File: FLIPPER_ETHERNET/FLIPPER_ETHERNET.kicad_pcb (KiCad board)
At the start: 2 copper layers, 67 x 25 mm, 38 parts, among them J1 RJ45_Hanrun_HR911105A_Horizon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, J2 Conn_01x08_Socket, J3 Conn_01x10_Socket, SW1 SW_Push, U1 ENC28J60x-ML, Y1 25MHz

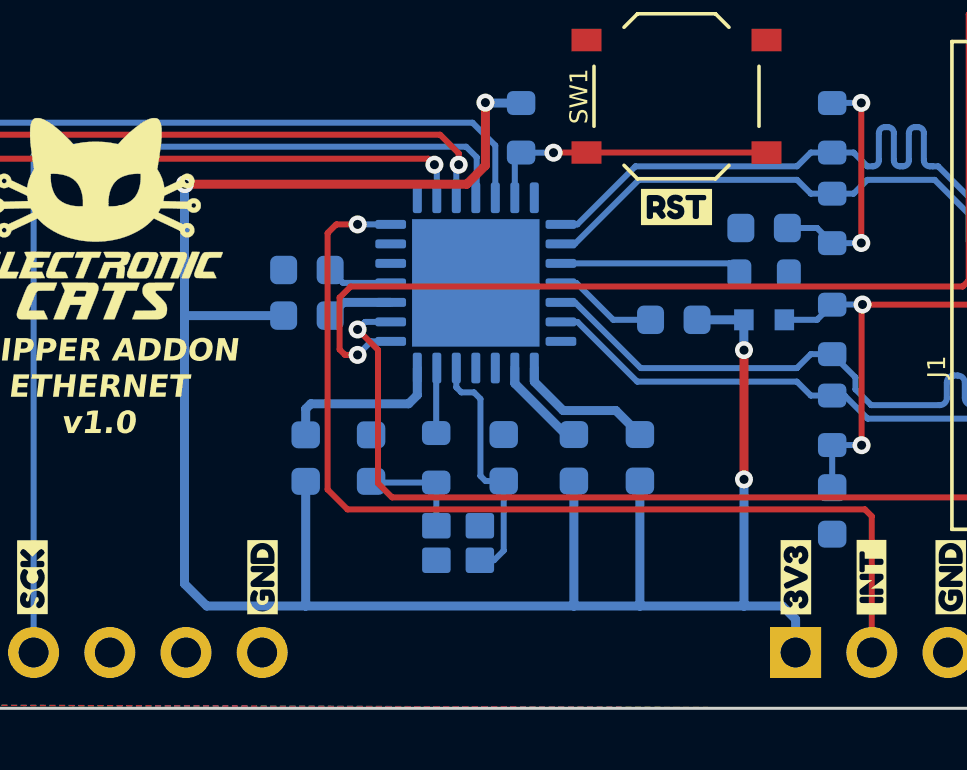
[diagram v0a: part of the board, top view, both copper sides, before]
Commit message: feat: some pcb routes corrected
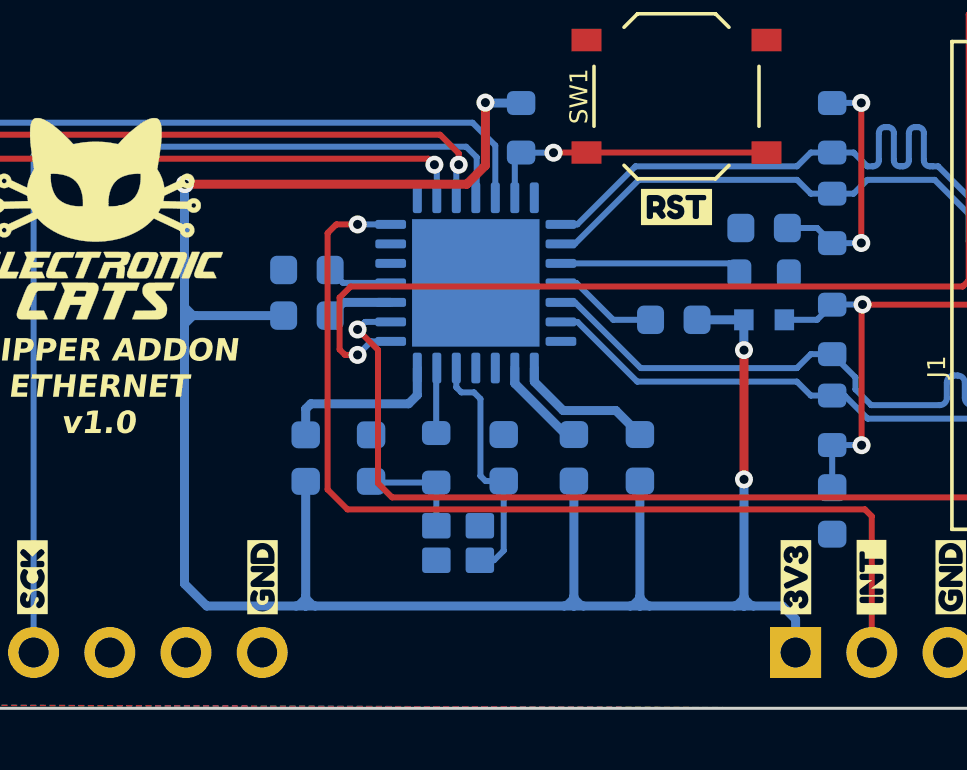
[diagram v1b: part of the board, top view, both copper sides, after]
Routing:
- net +3.3V: track 75.8 -> 80.4 mm
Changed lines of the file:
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@@
-	)
-	(segment
-		(start 150.63 62.555)
-		(end 150.63 66.72)
-		(width 0.3)
-		(layer "B.Cu")
-		(net 6)
 	)
 	(segment
@@
 	)
 	(segment
+		(start 150.63 66.4)
+		(end 150.31 66.72)
+		(width 0.2)
+		(layer "B.Cu")
+		(net 6)
+	)
+	(segment
+		(start 148.43 66.4)
+		(end 148.75 66.72)
+		(width 0.2)
+		(layer "B.Cu")
+		(net 6)
+	)
+	(segment
+		(start 148.43 66.4)
+		(end 148.43 66.72)
+		(width 0.3)
+		(layer "B.Cu")
+		(net 6)
+	)
+	(segment
 		(start 145.495 49.955)
 		(end 145.48 49.94)
@@
 	)
 	(segment
-		(start 154.1 62.5)
-		(end 154.1 66.72)
-		(width 0.3)
-		(layer "B.Cu")
-		(net 6)
-	)
-	(segment
 		(start 155.82 67.16)
 		(end 155.82 68.27)
@@
 	)
 	(segment
-		(start 139.49 62.565)
-		(end 139.49 66.72)
-		(width 0.3)
-		(layer "B.Cu")
-		(net 6)
-	)
-	(segment
-		(start 148.43 62.555)
-		(end 148.43 66.72)
-		(width 0.3)
+		(start 154.1 66.4)
+		(end 154.42 66.72)
+		(width 0.2)
 		(layer "B.Cu")
 		(net 6)
@@
 	)
 	(segment
+		(start 154.1 66.4)
+		(end 153.78 66.72)
+		(width 0.2)
+		(layer "B.Cu")
+		(net 6)
+	)
+	(segment
+		(start 135.45 57.04)
+		(end 135.45 57.39)
+		(width 0.3)
+		(layer "B.Cu")
+		(net 6)
+	)
+	(segment
+		(start 148.43 62.555)
+		(end 148.43 66.4)
+		(width 0.3)
+		(layer "B.Cu")
+		(net 6)
+	)
+	(segment
+		(start 148.43 66.4)
+		(end 148.11 66.72)
+		(width 0.2)
+		(layer "B.Cu")
+		(net 6)
+	)
+	(segment
 		(start 135.45 65.98)
 		(end 136.19 66.72)
@@
 	)
 	(segment
-		(start 154.1 66.72)
-		(end 155.38 66.72)
-		(width 0.3)
-		(layer "B.Cu")
-		(net 6)
-	)
-	(segment
-		(start 148.43 66.72)
-		(end 150.63 66.72)
+		(start 139.49 66.4)
+		(end 139.17 66.72)
+		(width 0.2)
+		(layer "B.Cu")
+		(net 6)
+	)
+	(segment
+		(start 139.49 66.4)
+		(end 139.49 66.72)
 		(width 0.3)
 		(layer "B.Cu")
@@
 	)
 	(segment
-		(start 136.19 66.72)
-		(end 139.49 66.72)
+		(start 139.81 66.72)
+		(end 148.11 66.72)
+		(width 0.3)
+		(layer "B.Cu")
+		(net 6)
+	)
+	(segment
+		(start 154.42 66.72)
+		(end 155.38 66.72)
+		(width 0.3)
+		(layer "B.Cu")
+		(net 6)
+	)
+	(segment
+		(start 148.11 66.72)
+		(end 148.43 66.72)
 		(width 0.3)
 		(layer "B.Cu")
@@
 	)
 	(segment
+		(start 150.63 66.72)
+		(end 150.95 66.72)
+		(width 0.3)
+		(layer "B.Cu")
+		(net 6)
+	)
+	(segment
 		(start 146.67 49.955)
 		(end 145.495 49.955)
@@
 	)
 	(segment
+		(start 135.8 57.04)
+		(end 135.45 57.04)
+		(width 0.3)
+		(layer "B.Cu")
+		(net 6)
+	)
+	(segment
+		(start 150.63 66.4)
+		(end 150.63 66.72)
+		(width 0.3)
+		(layer "B.Cu")
+		(net 6)
+	)
+	(segment
+		(start 153.78 66.72)
+		(end 154.1 66.72)
+		(width 0.3)
+		(layer "B.Cu")
+		(net 6)
+	)
+	(segment
+		(start 150.31 66.72)
+		(end 150.63 66.72)
+		(width 0.3)
+		(layer "B.Cu")
+		(net 6)
+	)
+	(segment
+		(start 150.63 66.4)
+		(end 150.95 66.72)
+		(width 0.2)
+		(layer "B.Cu")
+		(net 6)
+	)
+	(segment
+		(start 139.49 62.565)
+		(end 139.49 66.4)
+		(width 0.3)
+		(layer "B.Cu")
+		(net 6)
+	)
+	(segment
+		(start 148.43 66.72)
+		(end 148.75 66.72)
+		(width 0.3)
+		(layer "B.Cu")
+		(net 6)
+	)
+	(segment
+		(start 154.1 66.4)
+		(end 154.1 66.72)
+		(width 0.3)
+		(layer "B.Cu")
+		(net 6)
+	)
+	(segment
+		(start 135.8 57.04)
+		(end 135.45 56.69)
+		(width 0.2)
+		(layer "B.Cu")
+		(net 6)
+	)
+	(segment
+		(start 135.8 57.04)
+		(end 135.45 57.39)
+		(width 0.2)
+		(layer "B.Cu")
+		(net 6)
+	)
+	(segment
+		(start 135.45 56.69)
+		(end 135.45 57.04)
+		(width 0.3)
+		(layer "B.Cu")
+		(net 6)
+	)
+	(segment
+		(start 135.45 52.67)
+		(end 135.45 56.69)
+		(width 0.3)
+		(layer "B.Cu")
+		(net 6)
+	)
+	(segment
+		(start 150.63 62.555)
+		(end 150.63 66.4)
+		(width 0.3)
+		(layer "B.Cu")
+		(net 6)
+	)
+	(segment
+		(start 135.45 57.39)
+		(end 135.45 65.98)
+		(width 0.3)
+		(layer "B.Cu")
+		(net 6)
+	)
+	(segment
+		(start 148.75 66.72)
+		(end 150.31 66.72)
+		(width 0.3)
+		(layer "B.Cu")
+		(net 6)
+	)
+	(segment
 		(start 138.755 57.04)
-		(end 135.45 57.04)
-		(width 0.3)
-		(layer "B.Cu")
-		(net 6)
-	)
-	(segment
-		(start 150.63 66.72)
-		(end 154.1 66.72)
-		(width 0.3)
-		(layer "B.Cu")
-		(net 6)
-	)
-	(segment
-		(start 135.45 57.04)
-		(end 135.45 65.98)
+		(end 135.8 57.04)
+		(width 0.3)
+		(layer "B.Cu")
+		(net 6)
+	)
+	(segment
+		(start 154.1 62.5)
+		(end 154.1 66.4)
 		(width 0.3)
 		(layer "B.Cu")
@@
 	(segment
 		(start 139.49 66.72)
-		(end 148.43 66.72)
-		(width 0.3)
-		(layer "B.Cu")
-		(net 6)
-	)
-	(segment
-		(start 135.45 52.67)
-		(end 135.45 57.04)
-		(width 0.3)
-		(layer "B.Cu")
+		(end 139.81 66.72)
+		(width 0.3)
+		(layer "B.Cu")
+		(net 6)
+	)
+	(segment
+		(start 139.49 66.4)
+		(end 139.81 66.72)
+		(width 0.2)
+		(layer "B.Cu")
+		(net 6)
+	)
+	(segment
+		(start 154.1 66.72)
+		(end 154.42 66.72)
+		(width 0.3)
+		(layer "B.Cu")
+		(net 6)
+	)
+	(segment
+		(start 139.17 66.72)
+		(end 139.49 66.72)
+		(width 0.3)
+		(layer "B.Cu")
+		(net 6)
+	)
+	(segment
+		(start 150.95 66.72)
+		(end 153.78 66.72)
+		(width 0.3)
+		(layer "B.Cu")
+		(net 6)
+	)
+	(segment
+		(start 136.19 66.72)
+		(end 139.17 66.72)
+		(width 0.3)
+		(layer "B.Cu")
